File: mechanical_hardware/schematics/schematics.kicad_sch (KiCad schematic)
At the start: 19 parts, among them J1 Raspberry_Pi_4, J4 TB6612FNG, J5 Encoder, J6 Encoder, M1 Motor_DC, M2 Motor_DC, SW2 SW_DIP_x02, U1 5.1V, U2 5V, U3 11.5V, U4 ESP32-DevKitC, U5 MPU-9250, U6 MPU-6050

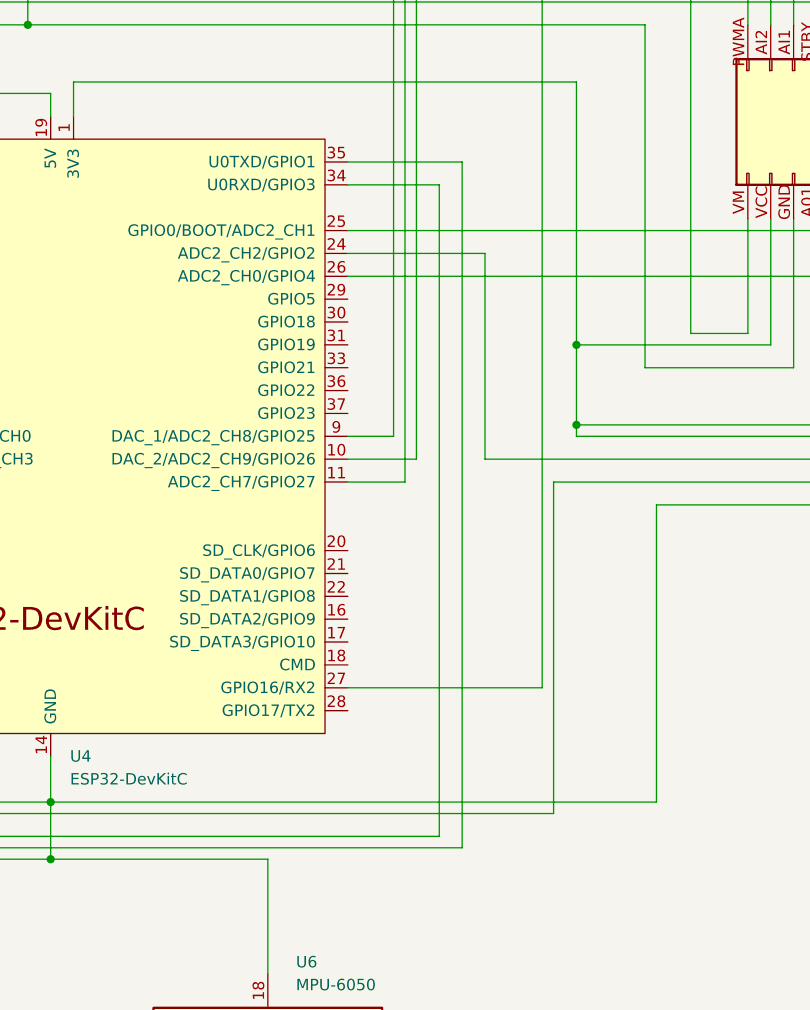
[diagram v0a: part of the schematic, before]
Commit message: schematics
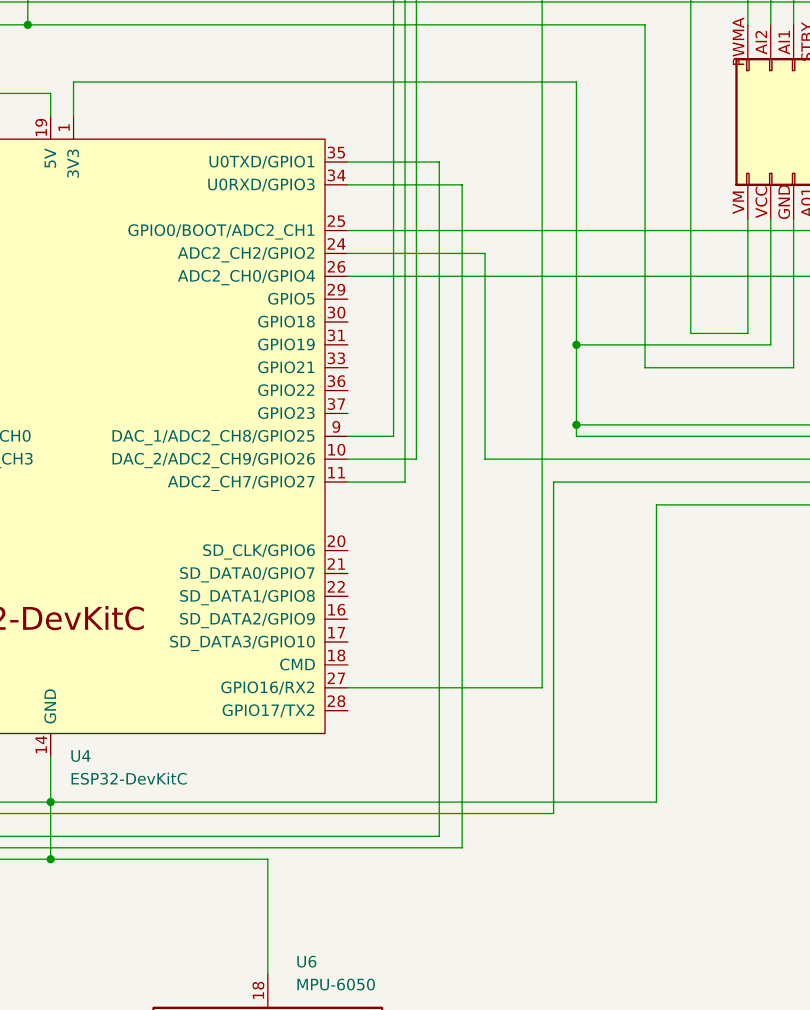
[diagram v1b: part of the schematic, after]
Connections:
- net at U4.34 (U0RXD/GPIO3): now also J1.8 (GPIO14/UART_TXD); no longer J1.10 (GPIO15/UART_RXD)
- net at U4.35 (U0TXD/GPIO1): now also J1.10 (GPIO15/UART_RXD); no longer J1.8 (GPIO14/UART_TXD)
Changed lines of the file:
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@@
+	(wire
+		(pts
+			(xy 246.38 146.05) (xy 246.38 220.98)
+		)
+		(stroke
+			(width 0)
+			(type default)
+		)
+	)
 	(wire
 		(pts
@@
 	(wire
 		(pts
-			(xy 246.38 148.59) (xy 236.22 148.59)
+			(xy 246.38 146.05) (xy 236.22 146.05)
 		)
 		(stroke
@@
 	(wire
 		(pts
-			(xy 248.92 222.25) (xy 248.92 146.05)
+			(xy 248.92 222.25) (xy 248.92 148.59)
 		)
 		(stroke
@@
 	(wire
 		(pts
-			(xy 236.22 146.05) (xy 248.92 146.05)
-		)
-		(stroke
-			(width 0)
-			(type default)
-		)
-	)
-	(wire
-		(pts
 			(xy 171.45 57.15) (xy 171.45 59.69)
 		)
@@
 	(wire
 		(pts
-			(xy 246.38 220.98) (xy 246.38 148.59)
-		)
-		(stroke
-			(width 0)
-			(type default)
-		)
-	)
-	(wire
-		(pts
 			(xy 285.75 124.46) (xy 243.84 124.46)
 		)
@@
 		)
 		(stroke
+			(width 0)
+			(type default)
+		)
+	)
+	(wire
+		(pts
+			(xy 236.22 148.59) (xy 248.92 148.59)
+		)
+		(stroke

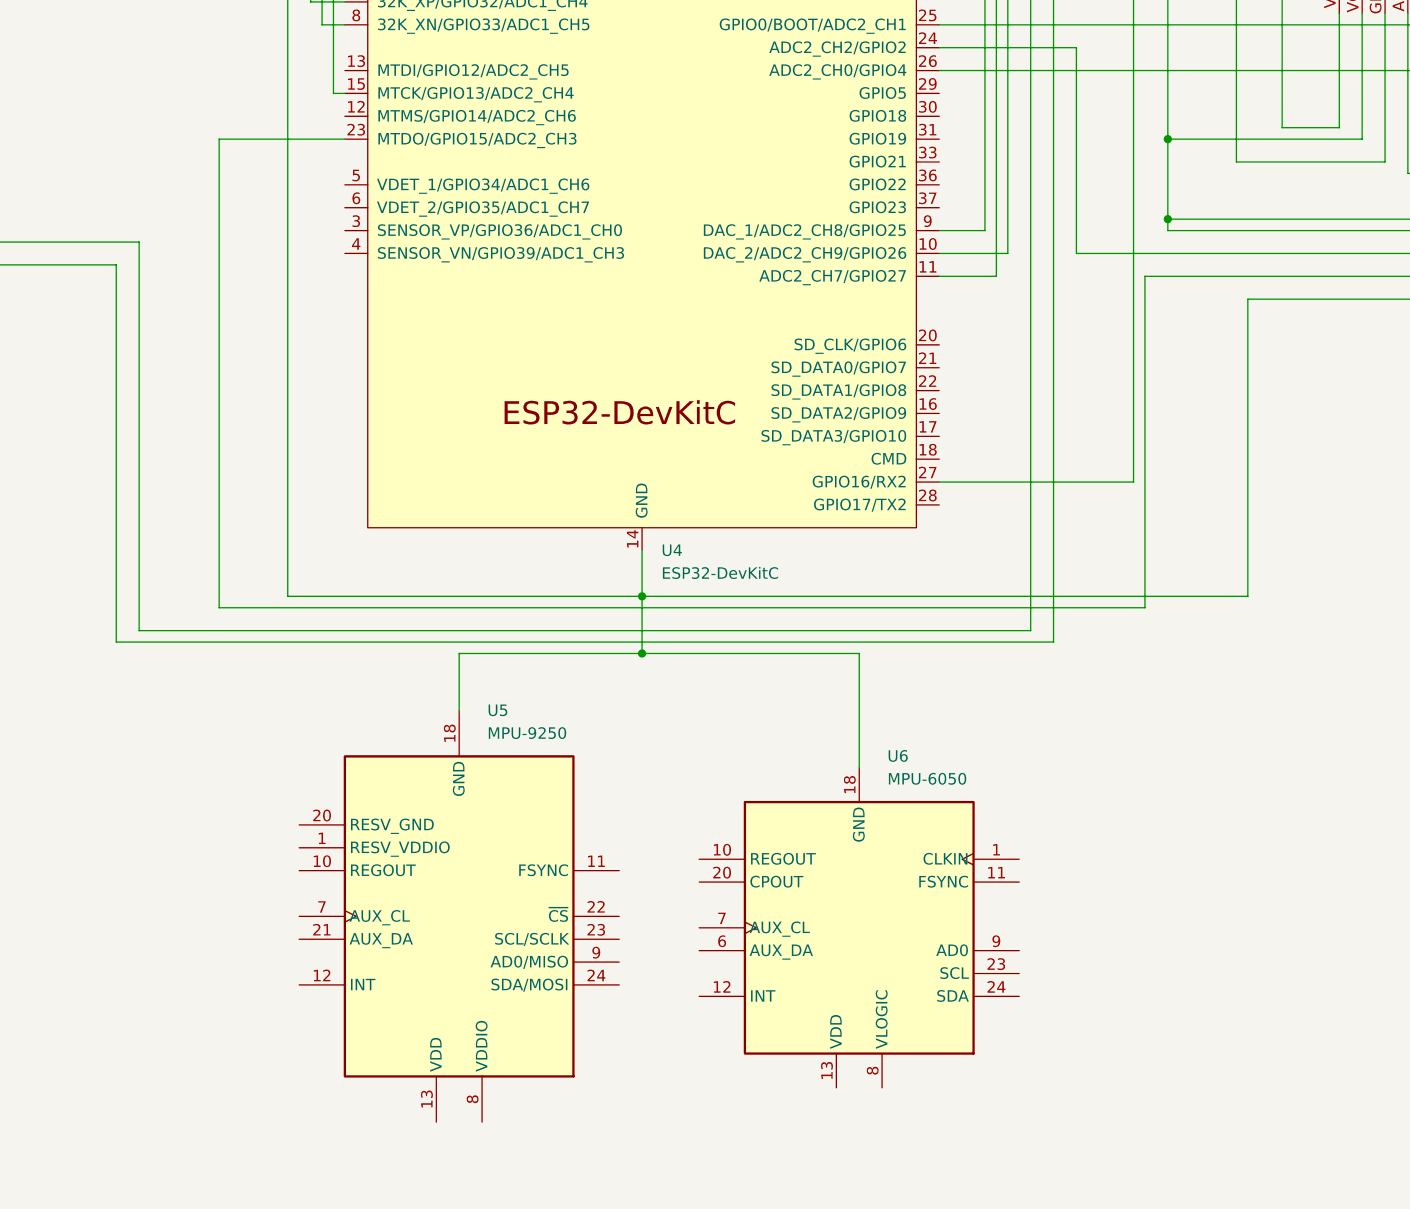
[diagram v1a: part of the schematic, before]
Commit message: schematics
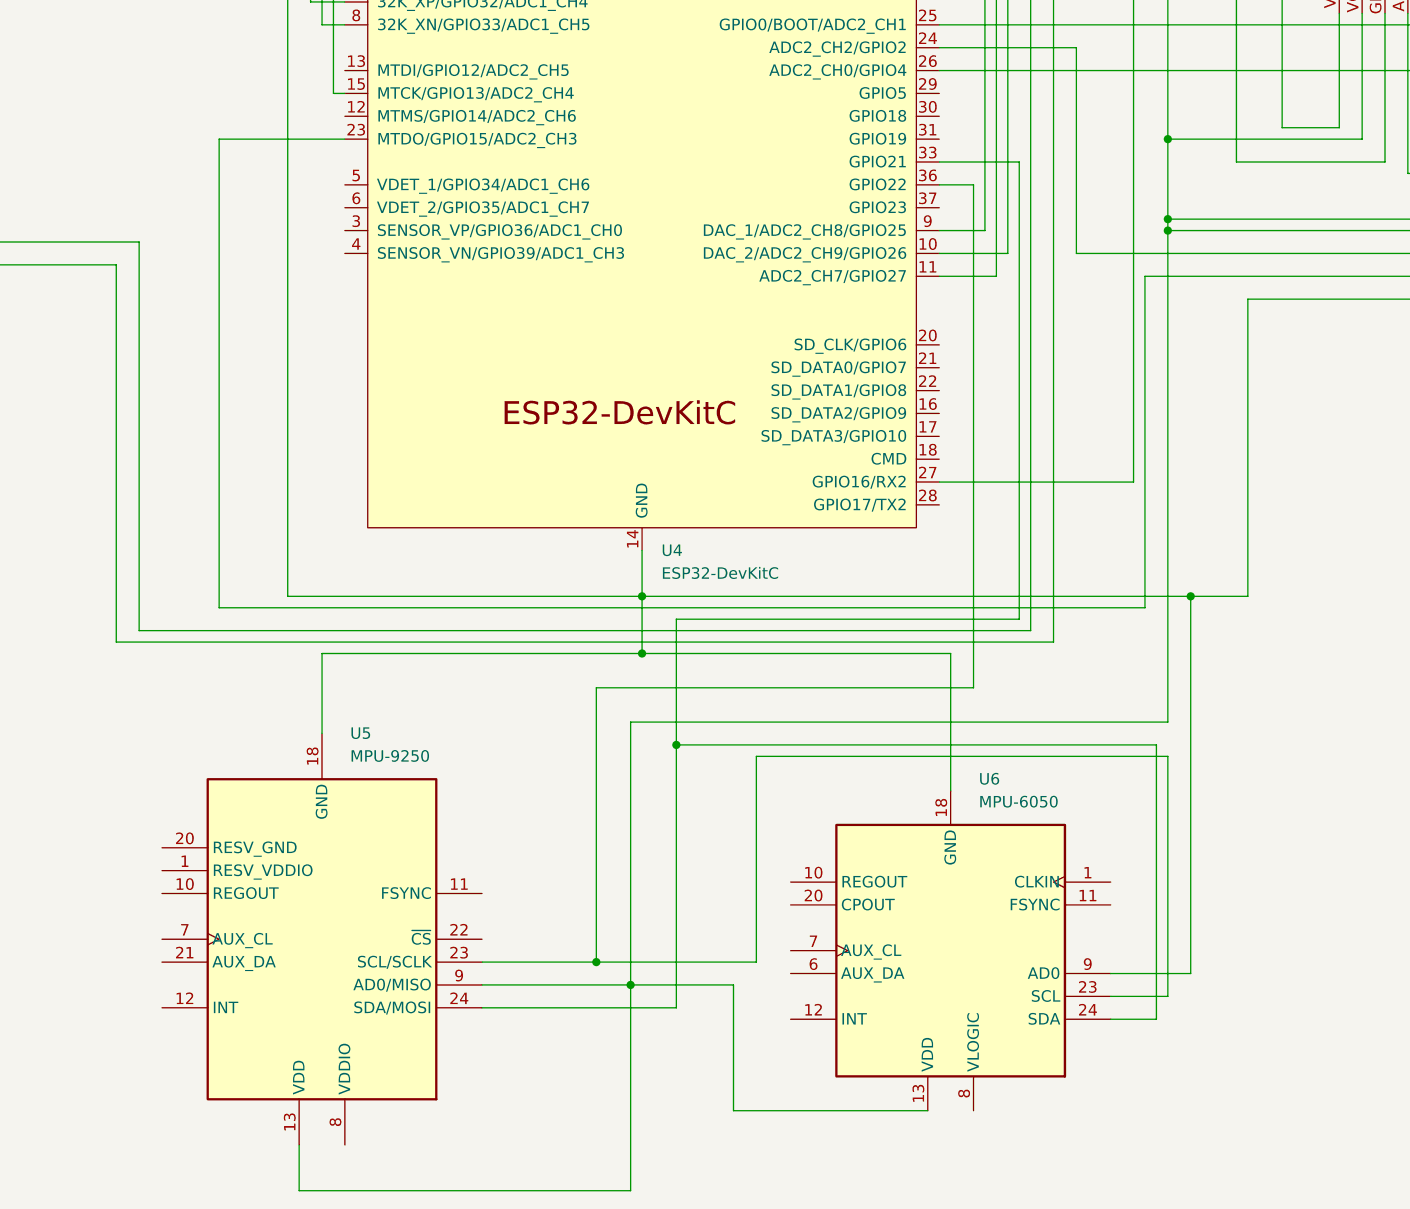
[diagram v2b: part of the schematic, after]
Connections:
- net at U6.13 (VDD): now also J4.VCC (Pin_2), J5.E-VCC (Pin_3), J6.E-VCC (Pin_3), U4.1 (3V3), U5.13 (VDD), U5.9 (AD0/MISO)
- net at J1.14 (GND), J1.20 (GND), J1.25 (GND)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: now also U6.9 (AD0)
- net at U6.23 (SCL): now also U4.36 (GPIO22), U5.23 (SCL/SCLK)
- net at U6.24 (SDA): now also U4.33 (GPIO21), U5.24 (SDA/MOSI)
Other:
- moved on the sheet: U5, U6
